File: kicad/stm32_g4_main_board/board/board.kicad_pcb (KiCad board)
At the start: 2 copper layers, 75 parts, among them Q1 CSD18514Q5A, Q10 CSD18514Q5A, Q11 CSD18514Q5A, Q12 CSD18514Q5A, Q13 CSD18514Q5A, Q14 CSD18514Q5A, Q15 CSD18514Q5A, Q16 CSD18514Q5A, Q17 CSD18514Q5A, Q18 CSD18514Q5A, Q2 CSD18514Q5A, Q3 CSD18514Q5A, Q4 CSD18514Q5A, Q5 CSD18514Q5A, Q6 CSD18514Q5A, Q7 CSD18514Q5A, Q8 CSD18514Q5A, Q9 CSD18514Q5A, U1 DRV8304HRHAR, U2 DRV8304HRHAR, U3 DRV8304HRHAR

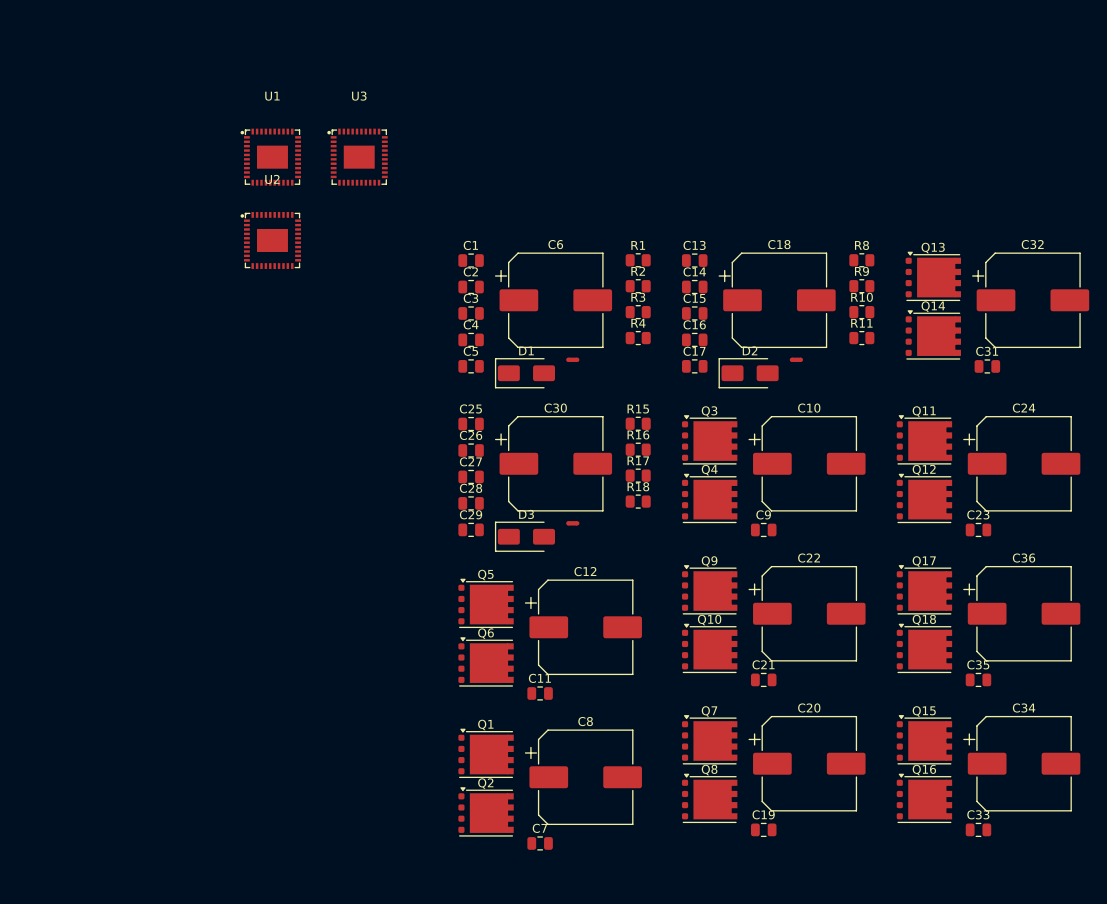
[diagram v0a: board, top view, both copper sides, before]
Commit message: V1 Board.
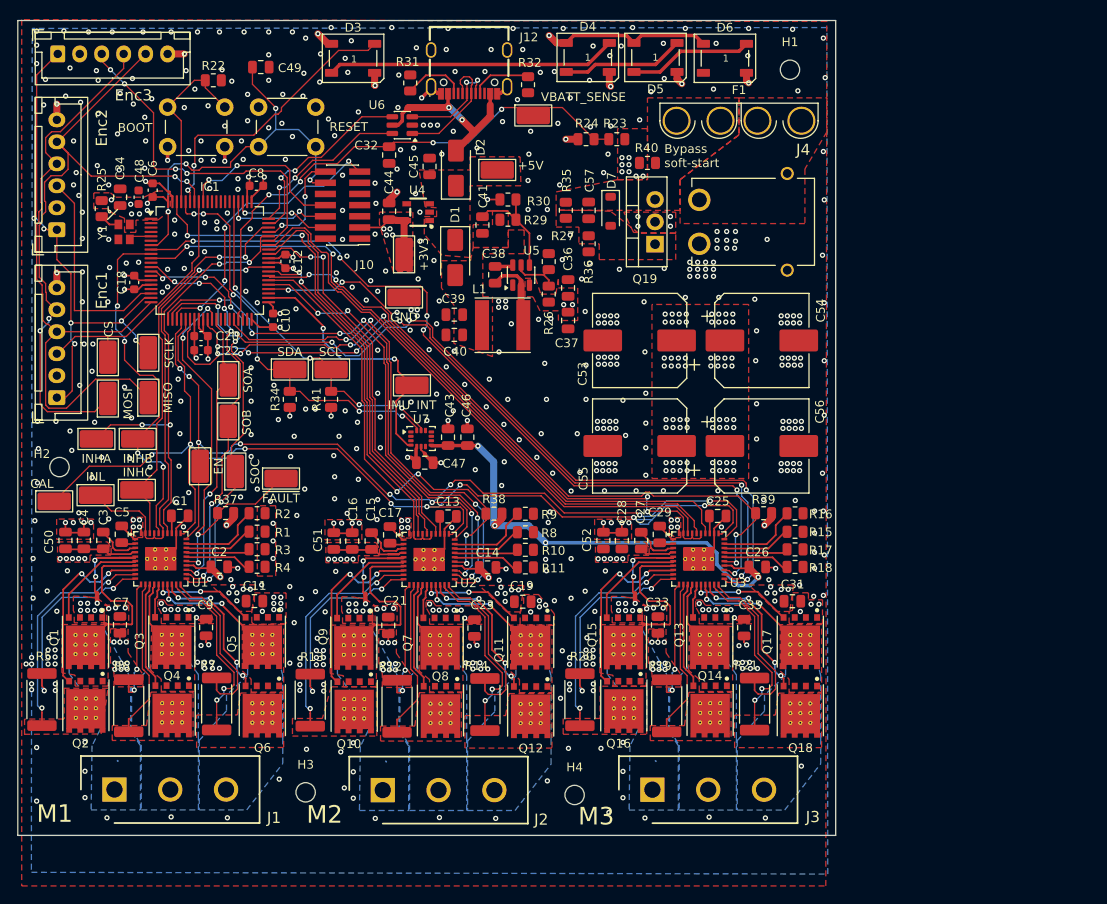
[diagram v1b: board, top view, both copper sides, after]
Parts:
- removed C24, C30: 150uF, Capacitor_SMD:CP_Elec_10x12.5
- added C37: 100n, Capacitor_SMD:C_0805_2012Metric, F.Cu at (78.3, 68.8)
- added C38: 100n, Capacitor_SMD:C_0805_2012Metric, F.Cu at (70.0, 63.6)
- added C39: 22u, Capacitor_SMD:C_0805_2012Metric, F.Cu at (65.3, 68.2)
- added C40: 22u, Capacitor_SMD:C_0805_2012Metric, F.Cu at (65.3, 70.5)
- added C41: 75p, Capacitor_SMD:C_0805_2012Metric, F.Cu at (68.5, 58.0)
- added C43: 100n, Capacitor_SMD:C_0805_2012Metric, F.Cu at (64.6, 82.1)
- added C44: 1u, Capacitor_SMD:C_0805_2012Metric, F.Cu at (57.9, 56.4)
- added C45: 1u, Capacitor_SMD:C_0805_2012Metric, F.Cu at (62.5, 51.3)
- added C46: 2u2, Capacitor_SMD:C_0805_2012Metric, F.Cu at (66.8, 82.1)
- added C47: 10n, Capacitor_SMD:C_0805_2012Metric, F.Cu at (62.0, 85.0)
- added C48: 100n, Capacitor_SMD:C_0603_1608Metric, F.Cu at (29.4, 54.8)
- added C49: 100n, Capacitor_SMD:C_0805_2012Metric, F.Cu at (43.3, 40.0)
- added C50: 10u, Capacitor_SMD:C_0805_2012Metric, F.Cu at (21.1, 93.8)
- added C51: 10u, Capacitor_SMD:C_0805_2012Metric, F.Cu at (51.6, 93.9)
- added C52: 10u, Capacitor_SMD:C_0805_2012Metric, F.Cu at (82.3, 93.9)
- added C53: 150u, Capacitor_SMD:CP_Elec_10x10.5, F.Cu at (86.4, 71.1)
- added C54: 150u, Capacitor_SMD:CP_Elec_10x10.5, F.Cu at (100.3, 71.1)
- added C55: 150u, Capacitor_SMD:CP_Elec_10x10.5, F.Cu at (86.4, 83.1)
- added C56: 150u, Capacitor_SMD:CP_Elec_10x10.5, F.Cu at (100.3, 83.1)
- added C57: 68n, Capacitor_SMD:C_0805_2012Metric, F.Cu at (80.6, 56.3)
- added D4: WS2812B, LED_SMD:LED_WS2812B_PLCC4_5.0x5.0mm_P3.2mm, F.Cu at (80.5, 38.9)
- added D5: WS2812B, LED_SMD:LED_WS2812B_PLCC4_5.0x5.0mm_P3.2mm, F.Cu at (88.2, 38.9)
- added D6: WS2812B, LED_SMD:LED_WS2812B_PLCC4_5.0x5.0mm_P3.2mm, F.Cu at (96.1, 39.0)
- added D7: 15V 0.5W, Diode_SMD:D_SOD-123, F.Cu at (83.1, 56.4)
- added F1: Fuse, jaguilar:Fuse_Blade_XF_507P, F.Cu at (97.7, 46.1)
- added H1: MountingHole, MountingHole:MountingHole_2.2mm_M2, F.Cu at (103.5, 40.3)
- added H2: MountingHole, MountingHole:MountingHole_2.2mm_M2, F.Cu at (20.4, 85.5)
- added H3: MountingHole, MountingHole:MountingHole_2.2mm_M2, F.Cu at (48.4, 122.5)
- added H4: MountingHole, MountingHole:MountingHole_2.2mm_M2, F.Cu at (79.0, 122.8)
- added IC1: STM32G474MET6TR, Package_QFP:LQFP-80_12x12mm_P0.5mm, F.Cu at (37.5, 62.0)
- added J1: MR30PW-M, jaguilar:PinHeader_01x03_Molex_6.35mm, F.Cu at (26.6, 122.2)
- added J10: STDC, Connector_PinHeader_1.27mm:PinHeader_2x07_P1.27mm_Vertical_SMD, F.Cu at (52.6, 55.7)
- added J11: JST-XH-B6B, Connector_JST:JST_XH_B6B-XH-A_1x06_P2.50mm_Vertical, F.Cu at (20.1, 77.6)
- added J12: USB_C_Receptacle_USB2, jaguilar:C165948_USB-C_SMD-TYPE-C-31-M-12_1, F.Cu at (67.0, 40.5)
- added J13: JST-XH-B6B, Connector_JST:JST_XH_B6B-XH-A_1x06_P2.50mm_Vertical, F.Cu at (20.1, 58.5)
- added J14: JST-XH-B6B, Connector_JST:JST_XH_B6B-XH-A_1x06_P2.50mm_Vertical, F.Cu at (20.2, 38.5)
- added J2: MR30PW-M, jaguilar:PinHeader_01x03_Molex_6.35mm, F.Cu at (57.2, 122.2)
- added J3: MR30PW-M, jaguilar:PinHeader_01x03_Molex_6.35mm, F.Cu at (87.8, 122.2)
- added J4: XT30PW-M, jaguilar:XT30PWM, F.Cu at (99.1, 57.6)
- added L1: 10u, Inductor_SMD:L_Taiyo-Yuden_NR-60xx, F.Cu at (70.8, 69.4)
- added Q19: IRF4905, Package_TO_SOT_THT:TO-220-3_Vertical, F.Cu at (88.2, 60.1)
- added R12: 7mOhm, jaguilar:R_2512_6332Metric_Kelvin, F.Cu at (58.8, 112.7)
- added R13: 7mOhm, jaguilar:R_2512_6332Metric_Kelvin, F.Cu at (48.9, 112.0)
- added R14: 7mOhm, jaguilar:R_2512_6332Metric_Kelvin, F.Cu at (68.8, 112.5)
- added R19: 7mOhm, jaguilar:R_2512_6332Metric_Kelvin, F.Cu at (89.5, 112.7)
- added R20: 7mOhm, jaguilar:R_2512_6332Metric_Kelvin, F.Cu at (79.6, 112.0)
- added R21: 7mOhm, jaguilar:R_2512_6332Metric_Kelvin, F.Cu at (99.5, 112.5)
- added R22: 10k, Resistor_SMD:R_0805_2012Metric, F.Cu at (37.9, 41.5)
- added R23: 82k, Resistor_SMD:R_0805_2012Metric, F.Cu at (83.8, 48.2)
- added R24: 10k, Resistor_SMD:R_0805_2012Metric, F.Cu at (80.3, 48.2)
- added R25: 10k, Resistor_SMD:R_0805_2012Metric, F.Cu at (25.2, 56.1)
- added R26: 511k, Resistor_SMD:R_0805_2012Metric, F.Cu at (76.1, 65.8)
- added R27: 105k, Resistor_SMD:R_0805_2012Metric, F.Cu at (76.1, 62.1)
- added R29: 100k, Resistor_SMD:R_0805_2012Metric, F.Cu at (71.4, 57.4)
- added R30: 13k3, Resistor_SMD:R_0805_2012Metric, F.Cu at (71.4, 55.1)
- added R31: 5k1, Resistor_SMD:R_0805_2012Metric, F.Cu at (60.3, 41.8)
- added R32: 5k1, Resistor_SMD:R_0805_2012Metric, F.Cu at (73.7, 42.0)
- added R34: 4k7, Resistor_SMD:R_0805_2012Metric, F.Cu at (46.6, 77.8)
- added R35: 100k, Resistor_SMD:R_0805_2012Metric, F.Cu at (78.0, 56.3)
- added R36: 150k, Resistor_SMD:R_0805_2012Metric, F.Cu at (80.6, 60.1)
- added R37: 10k, Resistor_SMD:R_0805_2012Metric, F.Cu at (39.3, 90.7)
- added R38: 10k, Resistor_SMD:R_0805_2012Metric, F.Cu at (69.8, 90.8)
- added R39: 10k, Resistor_SMD:R_0805_2012Metric, F.Cu at (100.5, 90.8)
- added R40: 0, Resistor_SMD:R_0805_2012Metric, F.Cu at (87.3, 50.9)
- added R41: 4k7, Resistor_SMD:R_0805_2012Metric, F.Cu at (51.3, 77.8)
- added R5: 7mOhm, jaguilar:R_2512_6332Metric_Kelvin, F.Cu at (18.4, 111.9)
- added R6: 7mOhm, jaguilar:R_2512_6332Metric_Kelvin, F.Cu at (28.3, 112.6)
- added R7: 7mOhm, jaguilar:R_2512_6332Metric_Kelvin, F.Cu at (38.3, 112.4)
- added SW1: BOOT, Button_Switch_THT:SW_PUSH_6mm_H5mm, F.Cu at (32.7, 44.5)
- added SW2: RESET, Button_Switch_THT:SW_PUSH_6mm_H5mm, F.Cu at (43.0, 44.5)
- added TP10: INHA, TestPoint:TestPoint_Keystone_5019_Miniature, F.Cu at (24.6, 82.3)
- added TP11: INHB, TestPoint:TestPoint_Keystone_5019_Miniature, F.Cu at (29.3, 82.3)
- added TP12: INHC, TestPoint:TestPoint_Keystone_5019_Miniature, F.Cu at (29.2, 88.1)
- added TP13: INL, TestPoint:TestPoint_Keystone_5019_Miniature, F.Cu at (24.5, 88.7)
- added TP14: SOA, TestPoint:TestPoint_Keystone_5019_Miniature, F.Cu at (39.6, 75.6)
- added TP15: SOB, TestPoint:TestPoint_Keystone_5019_Miniature, F.Cu at (39.6, 80.3)
- added TP16: SOC, TestPoint:TestPoint_Keystone_5019_Miniature, F.Cu at (40.4, 86.0)
- added TP17: CAL, TestPoint:TestPoint_Keystone_5019_Miniature, F.Cu at (19.8, 89.4)
- added TP18: +5V, TestPoint:TestPoint_Keystone_5019_Miniature, F.Cu at (70.2, 51.7)
- added TP19: +3V3, TestPoint:TestPoint_Keystone_5019_Miniature, F.Cu at (59.6, 61.3)
- added TP2: SCLK, TestPoint:TestPoint_Keystone_5019_Miniature, F.Cu at (30.5, 72.5)
- added TP20: GND, TestPoint:TestPoint_Keystone_5019_Miniature, F.Cu at (59.6, 66.2)
- added TP21: IMU_INT, TestPoint:TestPoint_Keystone_5019_Miniature, F.Cu at (60.5, 76.2)
- added TP22: VBATT_SENSE, TestPoint:TestPoint_Keystone_5019_Miniature, F.Cu at (74.3, 45.5)
- added TP3: MISO, TestPoint:TestPoint_Keystone_5019_Miniature, F.Cu at (30.5, 77.6)
- added TP4: MOSI, TestPoint:TestPoint_Keystone_5019_Miniature, F.Cu at (25.9, 77.7)
- added TP5: CS, TestPoint:TestPoint_Keystone_5019_Miniature, F.Cu at (25.9, 73.0)
- added TP6: SDA, TestPoint:TestPoint_Keystone_5019_Miniature, F.Cu at (46.6, 74.4)
- added TP7: SCL, TestPoint:TestPoint_Keystone_5019_Miniature, F.Cu at (51.3, 74.4)
- added TP8: EN, TestPoint:TestPoint_Keystone_5019_Miniature, F.Cu at (36.4, 85.4)
- added TP9: ~{FAULT}, TestPoint:TestPoint_Keystone_5019_Miniature, F.Cu at (45.6, 86.8)
- added U4: AP2112K-3.3TRG1(MS), jaguilar:C22365427_SOT-23-5_L2_9-W1_6-P0_95-LS2_7-BR, F.Cu at (61.2, 56.5)
- added U5: TPS54302, Package_TO_SOT_SMD:SOT-23-6, F.Cu at (72.9, 63.7)
- added U6: USBLC6-2SC6, Package_TO_SOT_SMD:SOT-23-6, F.Cu at (59.4, 46.6)
- added U7: ICM-42670-P, Package_LGA:LGA-14_3x2.5mm_P0.5mm_LayoutBorder3x4y, F.Cu at (61.5, 82.2)
- added Y1: SG-210STF_16.0000ML0, jaguilar:SG-210STF_EPS, F.Cu at (27.6, 58.6)
- C1, C13, C25: value 0.1 uF -> 1u
- C10, C12, C18, C20, C6, C8: value 150uF -> 100n; footprint Capacitor_SMD:CP_Elec_10x12.5 -> Capacitor_SMD:C_0603_1608Metric
- C11, C15, C19, C21, C23, C27, C3, C31, C33, C35, C7, C9: value 1uF -> 1u
- C14, C2, C26: value 1uF -> 100n
- C16, C28, C4: value 0.1 uF -> 100n
- C17, C29, C5: value 22nF -> 22n
- C22: value 150uF -> 1u; footprint Capacitor_SMD:CP_Elec_10x12.5 -> Capacitor_SMD:C_0603_1608Metric
- C32, C34: value 150uF -> 100n; footprint Capacitor_SMD:CP_Elec_10x12.5 -> Capacitor_SMD:C_0805_2012Metric
- C36: value 150uF -> 10u; footprint Capacitor_SMD:CP_Elec_10x12.5 -> Capacitor_SMD:C_0805_2012Metric
- D1, D2: value SMAJ18A -> SS14
- D3: value SMAJ18A -> WS2812B; footprint Diode_SMD:D_SMA -> LED_SMD:LED_WS2812B_PLCC4_5.0x5.0mm_P3.2mm
- Q1, Q10, Q11, Q12, Q13, Q14, Q15, Q16, Q17, Q18, Q2, Q3, Q4, Q5, Q6, Q7, Q8, Q9: footprint Package_SON:VSONP-8-1EP_5x6_P1.27mm -> jaguilar:CSD18514Q5A
- U1, U2, U3: footprint Local:C2677109_VQFN-40_L6_0-W6_0-P0_50-TL-EP -> jaguilar:C2677109_VQFN-40_L6_0-W6_0-P0_50-TL-EP
- moved C34 121.4 mm to (27.3, 54.8), turned to 90 degrees
- moved C20 84.6 mm to (36.5, 70.6), turned to 180 degrees
- moved C8 77.0 mm to (42.8, 53.5)
- moved C22 75.4 mm to (36.5, 72.2), turned to 180 degrees
- moved C32 75.1 mm to (57.9, 50.0), turned to -90 degrees
- moved C18 73.4 mm to (28.9, 64.5), turned to 90 degrees
- moved Q4 65.7 mm to (33.2, 113.1), turned to -90 degrees
- moved Q3 65.3 mm to (33.2, 105.3), turned to -90 degrees
- moved C9 64.4 mm to (37.1, 103.7), turned to 90 degrees
- moved C36 63.8 mm to (78.3, 65.1), turned to 90 degrees
- moved C10 63.1 mm to (44.7, 68.8), turned to -90 degrees
- moved NT1 60.5 mm to (24.7, 100.3), turned to -90 degrees
- moved U3 59.8 mm to (93.1, 96.0)
- moved C23 58.4 mm to (67.6, 103.8), turned to 90 degrees
- moved D3 57.9 mm to (53.8, 39.0)
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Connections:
- C10 pad 1: +BATT -> +3V3
- C12 pad 1: +BATT -> +3V3
- C15 pad 2: +3V3 -> Net-(U2-VCP)
- C18 pad 1: +BATT -> +3V3
- C20 pad 1: +BATT -> +3V3
- C22 pad 1: +BATT -> +3V3
- C27 pad 2: +3V3 -> Net-(U3-VCP)
- C3 pad 2: +3V3 -> Net-(U1-VCP)
- C32 pad 1: +BATT -> /Controller/VBATT_SENSE
- C34 pad 1: +BATT -> +3V3
- C6 pad 1: +BATT -> +3V3
- C8 pad 1: +BATT -> +3V3
- D1 pad 1: +BATT -> +5V
- D1 pad 2: GND -> /5V_REG
- D2 pad 1: +BATT -> +5V
- D2 pad 2: GND -> /USB_VBUS
- D3 pad 1: +BATT -> +3V3
- D3 pad 2: GND -> Net-(D3-DOUT)
- Q1 pad 1: /Motor Channel/half_bridge/Out -> +BATT
- Q1 pad 2: /Motor Channel/half_bridge/GateH -> +BATT
- Q10 pad 1: Net-(Q10-S) -> /mchan2/OUTA
- Q10 pad 2: /Motor Channel1/half_bridge/GateL -> /mchan2/OUTA
- Q10 pad 3: /Motor Channel1/half_bridge/Out -> /mchan2/OUTA
- Q11 pad 1: /Motor Channel1/half_bridge2/Out -> +BATT
- Q11 pad 2: /Motor Channel1/half_bridge2/GateH -> +BATT
- Q12 pad 1: Net-(Q12-S) -> /mchan2/OUTC
- Q12 pad 2: /Motor Channel1/half_bridge2/GateL -> /mchan2/OUTC
- Q12 pad 3: /Motor Channel1/half_bridge2/Out -> /mchan2/OUTC
- Q13 pad 1: /Motor Channel2/half_bridge1/Out -> +BATT
- Q13 pad 2: /Motor Channel2/half_bridge1/GateH -> +BATT
- Q14 pad 1: Net-(Q14-S) -> /mchan3/OUTB
- Q14 pad 2: /Motor Channel2/half_bridge1/GateL -> /mchan3/OUTB
- Q14 pad 3: /Motor Channel2/half_bridge1/Out -> /mchan3/OUTB
- Q15 pad 1: /Motor Channel2/half_bridge/Out -> +BATT
- Q15 pad 2: /Motor Channel2/half_bridge/GateH -> +BATT
- Q16 pad 1: Net-(Q16-S) -> /mchan3/OUTA
- Q16 pad 2: /Motor Channel2/half_bridge/GateL -> /mchan3/OUTA
- Q16 pad 3: /Motor Channel2/half_bridge/Out -> /mchan3/OUTA
- Q17 pad 1: /Motor Channel2/half_bridge2/Out -> +BATT
- Q17 pad 2: /Motor Channel2/half_bridge2/GateH -> +BATT
- Q18 pad 1: Net-(Q18-S) -> /mchan3/OUTC
- Q18 pad 2: /Motor Channel2/half_bridge2/GateL -> /mchan3/OUTC
- Q18 pad 3: /Motor Channel2/half_bridge2/Out -> /mchan3/OUTC
- Q2 pad 1: Net-(Q2-S) -> /mchan1/OUTA
- Q2 pad 2: /Motor Channel/half_bridge/GateL -> /mchan1/OUTA
- Q2 pad 3: /Motor Channel/half_bridge/Out -> /mchan1/OUTA
- Q3 pad 1: /Motor Channel/half_bridge1/Out -> +BATT
- Q3 pad 2: /Motor Channel/half_bridge1/GateH -> +BATT
- Q4 pad 1: Net-(Q4-S) -> /mchan1/OUTB
- Q4 pad 2: /Motor Channel/half_bridge1/GateL -> /mchan1/OUTB
- Q4 pad 3: /Motor Channel/half_bridge1/Out -> /mchan1/OUTB
- Q5 pad 1: /Motor Channel/half_bridge2/Out -> +BATT
- Q5 pad 2: /Motor Channel/half_bridge2/GateH -> +BATT
- Q6 pad 1: Net-(Q6-S) -> /mchan1/OUTC
- Q6 pad 2: /Motor Channel/half_bridge2/GateL -> /mchan1/OUTC
- Q6 pad 3: /Motor Channel/half_bridge2/Out -> /mchan1/OUTC
- Q7 pad 1: /Motor Channel1/half_bridge1/Out -> +BATT
- Q7 pad 2: /Motor Channel1/half_bridge1/GateH -> +BATT
- Q8 pad 1: Net-(Q8-S) -> /mchan2/OUTB
- Q8 pad 2: /Motor Channel1/half_bridge1/GateL -> /mchan2/OUTB
- Q8 pad 3: /Motor Channel1/half_bridge1/Out -> /mchan2/OUTB
- Q9 pad 1: /Motor Channel1/half_bridge/Out -> +BATT
- Q9 pad 2: /Motor Channel1/half_bridge/GateH -> +BATT
- U1 pad 10: /Motor Channel/half_bridge/ShuntL -> /mchan1/half_bridge/ShuntL
- U1 pad 11: /Motor Channel/half_bridge1/ShuntL -> /mchan1/half_bridge1/ShuntL
- U1 pad 12: /Motor Channel/half_bridge1/ShuntH -> /mchan1/half_bridge1/ShuntH
- U1 pad 13: /Motor Channel/half_bridge1/GateL -> /mchan1/half_bridge1/GateL
- U1 pad 14: /Motor Channel/half_bridge1/Out -> /mchan1/OUTB
- U1 pad 15: /Motor Channel/half_bridge1/GateH -> /mchan1/half_bridge1/GateH
- U1 pad 16: /Motor Channel/half_bridge2/GateH -> /mchan1/half_bridge2/GateH
- U1 pad 17: /Motor Channel/half_bridge2/Out -> /mchan1/OUTC
- U1 pad 18: /Motor Channel/half_bridge2/GateL -> /mchan1/half_bridge2/GateL
- U1 pad 19: /Motor Channel/half_bridge2/ShuntH -> /mchan1/half_bridge2/ShuntH
- U1 pad 20: /Motor Channel/half_bridge2/ShuntL -> /mchan1/half_bridge2/ShuntL
- U1 pad 25: /Controller/M1.nFAULT -> /Controller/M1.~{FAULT}
- U1 pad 3: +3V3 -> Net-(U1-VCP)
- U1 pad 30: /Controller/M1.EN -> /Controller/EN
- U1 pad 31: /Controller/M1.CAL -> /Controller/CAL
- U1 pad 6: /Motor Channel/half_bridge/GateH -> /mchan1/half_bridge/GateH
- U1 pad 7: /Motor Channel/half_bridge/Out -> /mchan1/OUTA
- U1 pad 8: /Motor Channel/half_bridge/GateL -> /mchan1/half_bridge/GateL
- U1 pad 9: /Motor Channel/half_bridge/ShuntH -> /mchan1/half_bridge/ShuntH
- U2 pad 10: /Motor Channel1/half_bridge/ShuntL -> /mchan2/half_bridge/ShuntL
- U2 pad 11: /Motor Channel1/half_bridge1/ShuntL -> /mchan2/half_bridge1/ShuntL
- U2 pad 12: /Motor Channel1/half_bridge1/ShuntH -> /mchan2/half_bridge1/ShuntH
- U2 pad 13: /Motor Channel1/half_bridge1/GateL -> /mchan2/half_bridge1/GateL
- U2 pad 14: /Motor Channel1/half_bridge1/Out -> /mchan2/OUTB
- U2 pad 15: /Motor Channel1/half_bridge1/GateH -> /mchan2/half_bridge1/GateH
- U2 pad 16: /Motor Channel1/half_bridge2/GateH -> /mchan2/half_bridge2/GateH
- U2 pad 17: /Motor Channel1/half_bridge2/Out -> /mchan2/OUTC
- U2 pad 18: /Motor Channel1/half_bridge2/GateL -> /mchan2/half_bridge2/GateL
- U2 pad 19: /Motor Channel1/half_bridge2/ShuntH -> /mchan2/half_bridge2/ShuntH
- U2 pad 20: /Motor Channel1/half_bridge2/ShuntL -> /mchan2/half_bridge2/ShuntL
- U2 pad 25: /Controller/M2.nFAULT -> /Controller/M2.~{FAULT}
- U2 pad 3: +3V3 -> Net-(U2-VCP)
- U2 pad 30: /Controller/M2.EN -> /Controller/EN
- U2 pad 31: /Controller/M2.CAL -> /Controller/CAL
- U2 pad 6: /Motor Channel1/half_bridge/GateH -> /mchan2/half_bridge/GateH
- U2 pad 7: /Motor Channel1/half_bridge/Out -> /mchan2/OUTA
- U2 pad 8: /Motor Channel1/half_bridge/GateL -> /mchan2/half_bridge/GateL
- U2 pad 9: /Motor Channel1/half_bridge/ShuntH -> /mchan2/half_bridge/ShuntH
- U3 pad 10: /Motor Channel2/half_bridge/ShuntL -> /mchan3/half_bridge/ShuntL
- U3 pad 11: /Motor Channel2/half_bridge1/ShuntL -> /mchan3/half_bridge1/ShuntL
- U3 pad 12: /Motor Channel2/half_bridge1/ShuntH -> /mchan3/half_bridge1/ShuntH
- U3 pad 13: /Motor Channel2/half_bridge1/GateL -> /mchan3/half_bridge1/GateL
- U3 pad 14: /Motor Channel2/half_bridge1/Out -> /mchan3/OUTB
- U3 pad 15: /Motor Channel2/half_bridge1/GateH -> /mchan3/half_bridge1/GateH
- U3 pad 16: /Motor Channel2/half_bridge2/GateH -> /mchan3/half_bridge2/GateH
- U3 pad 17: /Motor Channel2/half_bridge2/Out -> /mchan3/OUTC
- U3 pad 18: /Motor Channel2/half_bridge2/GateL -> /mchan3/half_bridge2/GateL
- U3 pad 19: /Motor Channel2/half_bridge2/ShuntH -> /mchan3/half_bridge2/ShuntH
- U3 pad 20: /Motor Channel2/half_bridge2/ShuntL -> /mchan3/half_bridge2/ShuntL
- U3 pad 25: /Controller/M3.nFAULT -> /Controller/M3.~{FAULT}
- U3 pad 3: +3V3 -> Net-(U3-VCP)
- U3 pad 30: /Controller/M3.EN -> /Controller/EN
- U3 pad 31: /Controller/M3.CAL -> /Controller/CAL
- U3 pad 6: /Motor Channel2/half_bridge/GateH -> /mchan3/half_bridge/GateH
- U3 pad 7: /Motor Channel2/half_bridge/Out -> /mchan3/OUTA
- U3 pad 8: /Motor Channel2/half_bridge/GateL -> /mchan3/half_bridge/GateL
- U3 pad 9: /Motor Channel2/half_bridge/ShuntH -> /mchan3/half_bridge/ShuntH
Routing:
- net +3V3: track 0.00 -> 152.4 mm, vias 0 -> 33
- net /Controller/CAL: track 0.00 -> 128.5 mm, vias 0 -> 8
- net /Controller/EN: track 0.00 -> 108.1 mm, vias 0 -> 9
- net /Controller/M3.SOC: track 0.00 -> 94.9 mm, vias 0 -> 6
- net /Controller/M3.SOA: track 0.00 -> 94.1 mm, vias 0 -> 6
- net /Controller/M3.SOB: track 0.00 -> 86.6 mm, vias 0 -> 6
- net GND: track 0.00 -> 82.6 mm, vias 0 -> 619
- net /Controller/M3.INHB: track 0.00 -> 79.0 mm, vias 0 -> 2
- net /Controller/M3.INHA: track 0.00 -> 78.1 mm, vias 0 -> 4
- net /SPI1.MOSI: track 0.00 -> 76.5 mm, vias 0 -> 4
- net /Controller/M3.~{FAULT}: track 0.00 -> 76.2 mm, vias 0 -> 4
- net /SPI1.MISO: track 0.00 -> 73.7 mm
- net /Controller/M3.INHC: track 0.00 -> 66.3 mm
- net /Controller/M3.INL: track 0.00 -> 66.0 mm, vias 0 -> 4
- net /Controller/M2.SOB: track 0.00 -> 65.7 mm, vias 0 -> 6
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- added copper zone on F.Cu, net +3V3
- added copper zone on In2.Cu, net +3V3
- added copper zone on F.Cu, net +5V
- added copper zone on F.Cu, net +BATT
- added copper zone on In2.Cu, net +BATT
- added copper zone on F.Cu, net /5V_REG
- added copper zone on B.Cu, net /mchan1/OUTA
- added copper zone on F.Cu, net /mchan1/OUTA
- added copper zone on B.Cu, net /mchan1/OUTB
- added copper zone on F.Cu, net /mchan1/OUTB
- added copper zone on B.Cu, net /mchan1/OUTC
- added copper zone on F.Cu, net /mchan1/OUTC
- added copper zone on B.Cu, net /mchan2/OUTA
- added copper zone on F.Cu, net /mchan2/OUTA
- added copper zone on B.Cu, net /mchan2/OUTB
- added copper zone on F.Cu, net /mchan2/OUTB
- added copper zone on B.Cu, net /mchan2/OUTC
- added copper zone on F.Cu, net /mchan2/OUTC
- added copper zone on B.Cu, net /mchan3/OUTA
- added copper zone on F.Cu, net /mchan3/OUTA
- added copper zone on B.Cu, net /mchan3/OUTB
- added copper zone on F.Cu, net /mchan3/OUTB
- added copper zone on B.Cu, net /mchan3/OUTC
- added copper zone on F.Cu, net /mchan3/OUTC
- added copper zone on B.Cu, net GND
- added copper zone on F.Cu, net GND
- added copper zone on In1.Cu, net GND
- added copper zone on F.Cu, net Net-(D7-A)
- added copper zone on F.Cu, net Net-(D7-K)
- added copper zone on F.Cu, net Net-(J4-+)
- added copper zone on F.Cu, net Net-(Q10-S)
- added copper zone on F.Cu, net Net-(Q12-S)
- added copper zone on F.Cu, net Net-(Q14-S)
- added copper zone on F.Cu, net Net-(Q16-S)
- added copper zone on F.Cu, net Net-(Q18-S)
- added copper zone on F.Cu, net Net-(Q2-S)
- added copper zone on F.Cu, net Net-(Q4-S)
- added copper zone on F.Cu, net Net-(Q6-S)
- added copper zone on F.Cu, net Net-(Q8-S)
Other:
- board outline added: 93 x 92.7 mm
- copper layers 2 -> 4
- board text added: "AGUILAR HEAVY INDUSTRY Self Balancing Cube Control Board v0.2 2026-08"
- board text added: "Bypass soft-start"
- board text added: "M1"
- board text added: "M2"
- board text added: "M3"

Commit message: WIP - v2 board
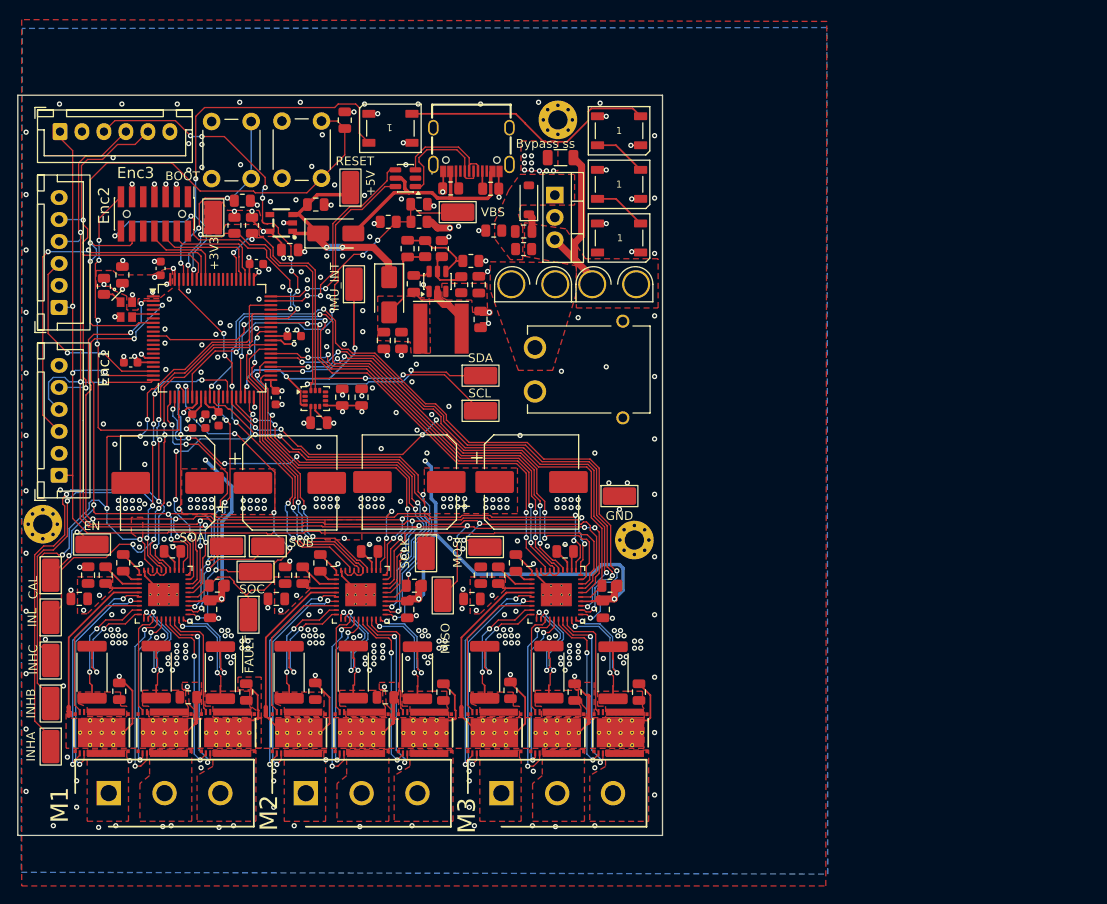
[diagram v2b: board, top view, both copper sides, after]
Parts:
- removed C10, C12, C18, C20, C48, C6, C8: 100n, Capacitor_SMD:C_0603_1608Metric
- removed C22: 1u, Capacitor_SMD:C_0603_1608Metric
- removed H3: MountingHole, MountingHole:MountingHole_2.2mm_M2
- removed IC1: STM32G474MET6TR, Package_QFP:LQFP-80_12x12mm_P0.5mm
- removed Q1, Q10, Q11, Q12, Q13, Q14, Q15, Q16, Q17, Q18, Q2, Q3, Q4, Q5, Q6, Q7, Q8, Q9: CSD18514Q5A, jaguilar:CSD18514Q5A
- removed R1, R15, R8: 75k, Resistor_SMD:R_0805_2012Metric
- removed R10, R17, R3: 18k, Resistor_SMD:R_0805_2012Metric
- removed R11, R18, R4: 47k, Resistor_SMD:R_0805_2012Metric
- removed R16, R2, R9: 45k, Resistor_SMD:R_0805_2012Metric
- removed TP5: CS, TestPoint:TestPoint_Keystone_5019_Miniature
- removed U1, U2, U3: DRV8304HRHAR, jaguilar:C2677109_VQFN-40_L6_0-W6_0-P0_50-TL-EP
- added C24: 100n, Capacitor_SMD:C_0603_1608Metric, F.Cu at (35.5, 80.3)
- added C30: 1u, Capacitor_SMD:C_0603_1608Metric, F.Cu at (37.0, 80.3)
- added C42: 100n, Capacitor_SMD:C_0603_1608Metric, F.Cu at (42.8, 62.4)
- added C58: 100n, Capacitor_SMD:C_0603_1608Metric, F.Cu at (28.5, 73.6)
- added C59: 100n, Capacitor_SMD:C_0603_1608Metric, F.Cu at (47.1, 70.6)
- added C60: 100n, Capacitor_SMD:C_0603_1608Metric, F.Cu at (45.0, 77.6)
- added C61: 100n, Capacitor_SMD:C_0603_1608Metric, F.Cu at (31.9, 62.9)
- added C62: 100n, Capacitor_SMD:C_0603_1608Metric, F.Cu at (38.5, 80.0)
- added U10: CSD88584Q5DC, jaguilar:DMM0022A, F.Cu at (39.5, 115.7)
- added U11: CSD88584Q5DC, jaguilar:DMM0022A, F.Cu at (54.8, 115.7)
- added U12: CSD88584Q5DC, jaguilar:DMM0022A, F.Cu at (47.6, 115.7)
- added U13: CSD88584Q5DC, jaguilar:DMM0022A, F.Cu at (62.0, 115.7)
- added U14: CSD88584Q5DC, jaguilar:DMM0022A, F.Cu at (77.0, 115.7)
- added U15: CSD88584Q5DC, jaguilar:DMM0022A, F.Cu at (69.9, 115.7)
- added U16: CSD88584Q5DC, jaguilar:DMM0022A, F.Cu at (84.2, 115.7)
- added U17: STM32G474METx, Package_QFP:LQFP-80_12x12mm_P0.5mm, F.Cu at (37.8, 70.8)
- added U18: DRV8304SRHAR, jaguilar:QFN-40_EP_6.15x6.15_Pitch0.5mm, F.Cu at (32.2, 100.0)
- added U19: DRV8304SRHAR, jaguilar:QFN-40_EP_6.15x6.15_Pitch0.5mm, F.Cu at (54.7, 100.0)
- added U20: DRV8304SRHAR, jaguilar:QFN-40_EP_6.15x6.15_Pitch0.5mm, F.Cu at (76.9, 100.0)
- added U8: CSD88584Q5DC, jaguilar:DMM0022A, F.Cu at (25.2, 115.7)
- added U9: CSD88584Q5DC, jaguilar:DMM0022A, F.Cu at (32.4, 115.7)
- D7: value 15V 0.5W -> 10V 0.5W
- H1, H2, H4: footprint MountingHole:MountingHole_2.2mm_M2 -> MountingHole:MountingHole_2.2mm_M2_Pad_Via
- J10: footprint Connector_PinHeader_1.27mm:PinHeader_2x07_P1.27mm_Vertical_SMD -> jaguilar:FTSH-107-01-L-DV-K-A
- R40: footprint Resistor_SMD:R_0805_2012Metric -> Resistor_SMD:R_1206_3216Metric
- TP22: value VBATT_SENSE -> VBS
- moved H4 76.8 mm to (77.1, 46.0)
- moved H1 56.4 mm to (85.8, 93.8)
- moved C53 56.1 mm to (32.7, 87.3)
- moved C54 56.1 mm to (46.6, 87.3)
- moved TP4 46.1 mm to (68.8, 94.6), turned to 0 degrees
- moved TP3 40.4 mm to (64.0, 100.1), turned to -90 degrees
- moved TP2 39.0 mm to (62.1, 95.3), turned to -90 degrees
- moved TP10 35.4 mm to (19.4, 117.3), turned to -90 degrees
- moved TP20 33.3 mm to (84.1, 88.8)
- moved TP11 31.7 mm to (19.4, 112.4), turned to -90 degrees
- moved C31 26.8 mm to (79.0, 111.1), turned to 90 degrees
- moved C55 26.5 mm to (60.2, 87.2)
- moved C56 26.5 mm to (74.1, 87.2)
- moved F1 26.4 mm to (78.9, 64.7), turned to 180 degrees
- moved J4 25.1 mm to (80.4, 74.4)
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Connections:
- C11 pad 1: GND -> Net-(U10-PGND)
- C19 pad 1: GND -> Net-(U11-PGND)
- C21 pad 1: GND -> Net-(U12-PGND)
- C23 pad 1: GND -> Net-(U13-PGND)
- C31 pad 1: GND -> Net-(U14-PGND)
- C33 pad 1: GND -> Net-(U15-PGND)
- C35 pad 1: GND -> Net-(U16-PGND)
- C7 pad 1: GND -> Net-(U8-PGND)
- C9 pad 1: GND -> Net-(U9-PGND)
- R12 pad 1: Net-(Q8-S) -> Net-(U11-PGND)
- R13 pad 1: Net-(Q10-S) -> Net-(U12-PGND)
- R14 pad 1: Net-(Q12-S) -> Net-(U13-PGND)
- R19 pad 1: Net-(Q14-S) -> Net-(U14-PGND)
- R20 pad 1: Net-(Q16-S) -> Net-(U15-PGND)
- R21 pad 1: Net-(Q18-S) -> Net-(U16-PGND)
- R5 pad 1: Net-(Q2-S) -> Net-(U8-PGND)
- R6 pad 1: Net-(Q4-S) -> Net-(U9-PGND)
- R7 pad 1: Net-(Q6-S) -> Net-(U10-PGND)
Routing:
- net /SPI1.MISO: track 73.7 -> 163.9 mm, vias 0 -> 11
- net /SPI1.MOSI: track 76.5 -> 162.5 mm, vias 4 -> 8
- net /SPI1.SCLK: track 59.7 -> 139.8 mm, vias 6 -> 3
- net +BATT: track 25.3 -> 85.7 mm, vias 158 -> 55
- net /Controller/M3.~{CS}: track 0.00 -> 54.4 mm, vias 0 -> 4
- net /Controller/M2.~{CS}: track 0.00 -> 38.9 mm, vias 0 -> 2
- net /Controller/M3.SOA: track 94.1 -> 61.3 mm, vias 6 -> 4
- net /Controller/M1.INHA: track 51.5 -> 82.5 mm, vias 4 -> 5
- net /Controller/M1.~{CS}: track 0.00 -> 29.8 mm, vias 0 -> 4
- net +3V3: track 152.4 -> 125.2 mm, vias 33 -> 30
- net /Controller/M1.INHC: track 45.1 -> 72.2 mm, vias 2 -> 5
- net +5V: track 0.00 -> 26.1 mm, vias 0 -> 2
- net /Controller/M1.INHB: track 42.3 -> 68.2 mm, vias 4 -> 7
- net /Controller/~{RESET}: track 44.4 -> 69.5 mm, vias 4 -> 2
- net /mchan2/half_bridge/SourceH: track 0.00 -> 24.8 mm, vias 0 -> 2
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- added copper zone on F.Cu, net Net-(U10-PGND)
- added copper zone on F.Cu, net Net-(U11-PGND)
- added copper zone on F.Cu, net Net-(U12-PGND)
- added copper zone on F.Cu, net Net-(U13-PGND)
- added copper zone on F.Cu, net Net-(U14-PGND)
- added copper zone on F.Cu, net Net-(U15-PGND)
- added copper zone on F.Cu, net Net-(U16-PGND)
- added copper zone on F.Cu, net Net-(U8-PGND)
- added copper zone on F.Cu, net Net-(U9-PGND)
- removed copper zone on F.Cu, net +5V
- removed copper zone on B.Cu, net /mchan1/OUTA
- removed copper zone on B.Cu, net /mchan1/OUTB
- removed copper zone on B.Cu, net /mchan1/OUTC
- removed copper zone on B.Cu, net /mchan2/OUTA
- removed copper zone on B.Cu, net /mchan2/OUTB
- removed copper zone on B.Cu, net /mchan2/OUTC
- removed copper zone on B.Cu, net /mchan3/OUTA
- removed copper zone on B.Cu, net /mchan3/OUTB
- removed copper zone on B.Cu, net /mchan3/OUTC
- removed copper zone on F.Cu, net Net-(Q10-S)
- removed copper zone on F.Cu, net Net-(Q12-S)
- removed copper zone on F.Cu, net Net-(Q14-S)
- removed copper zone on F.Cu, net Net-(Q16-S)
- removed copper zone on F.Cu, net Net-(Q18-S)
- removed copper zone on F.Cu, net Net-(Q2-S)
- removed copper zone on F.Cu, net Net-(Q4-S)
- removed copper zone on F.Cu, net Net-(Q6-S)
- removed copper zone on F.Cu, net Net-(Q8-S)
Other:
- board size 93 x 92.7 mm -> 73.3 x 84.2 mm
- board text added: "AGUILAR HEAVY INDUSTRY Self Balancing Cube Control Board v0.3 2026-10"
- board text added: "Bypass ss"
- board text removed: "AGUILAR HEAVY INDUSTRY Self Balancing Cube Control Board v0.2 2026-08"
- board text removed: "Bypass soft-start"
